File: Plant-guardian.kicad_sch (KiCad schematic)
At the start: 6 parts

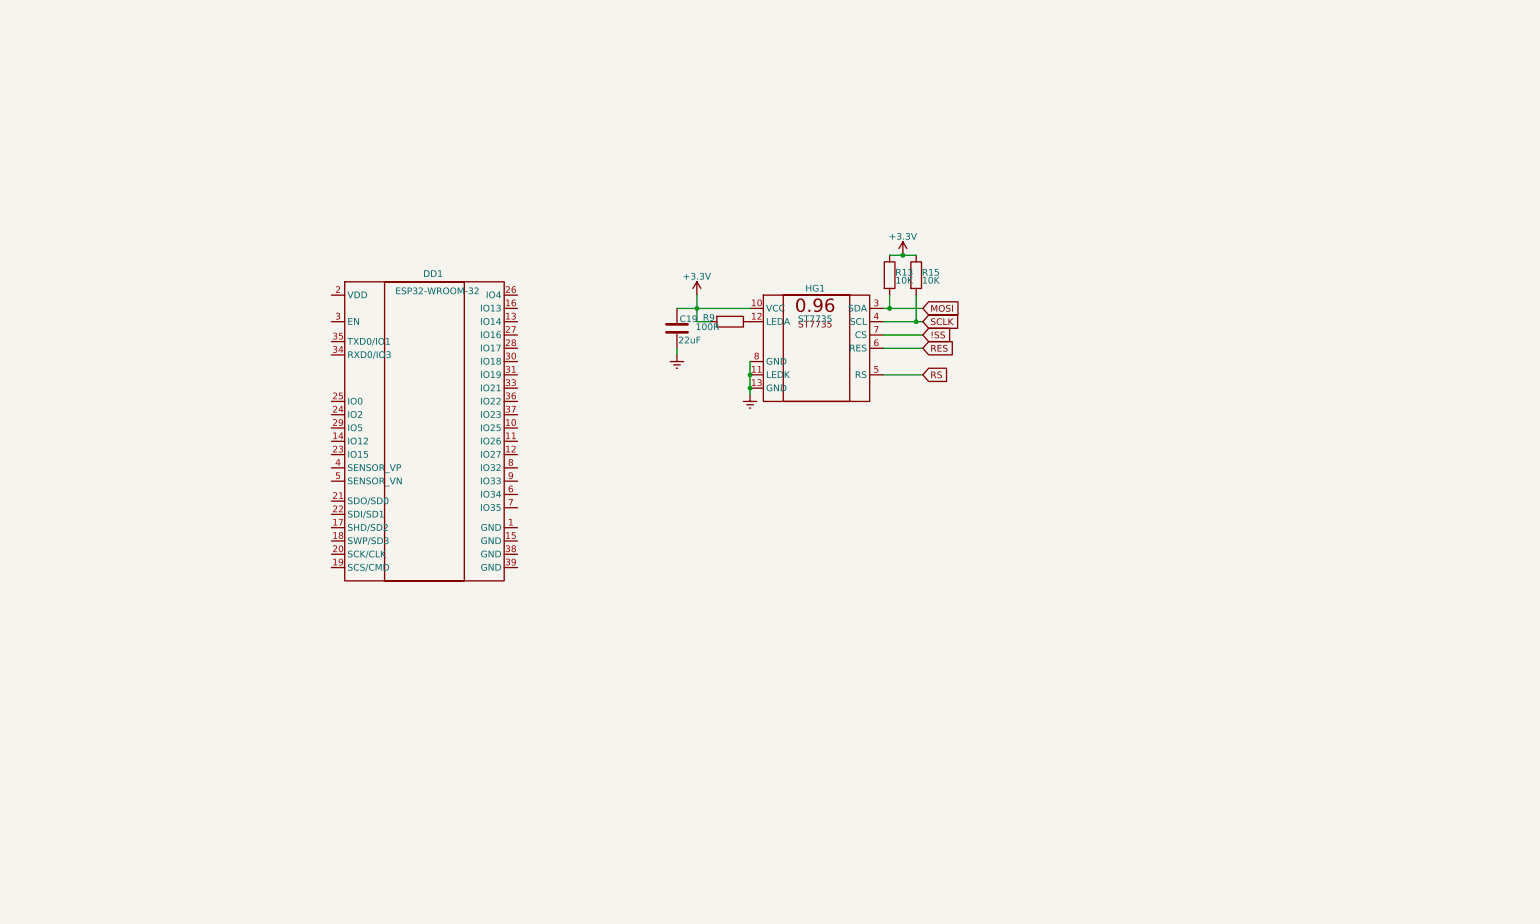
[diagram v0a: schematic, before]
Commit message: upd sch
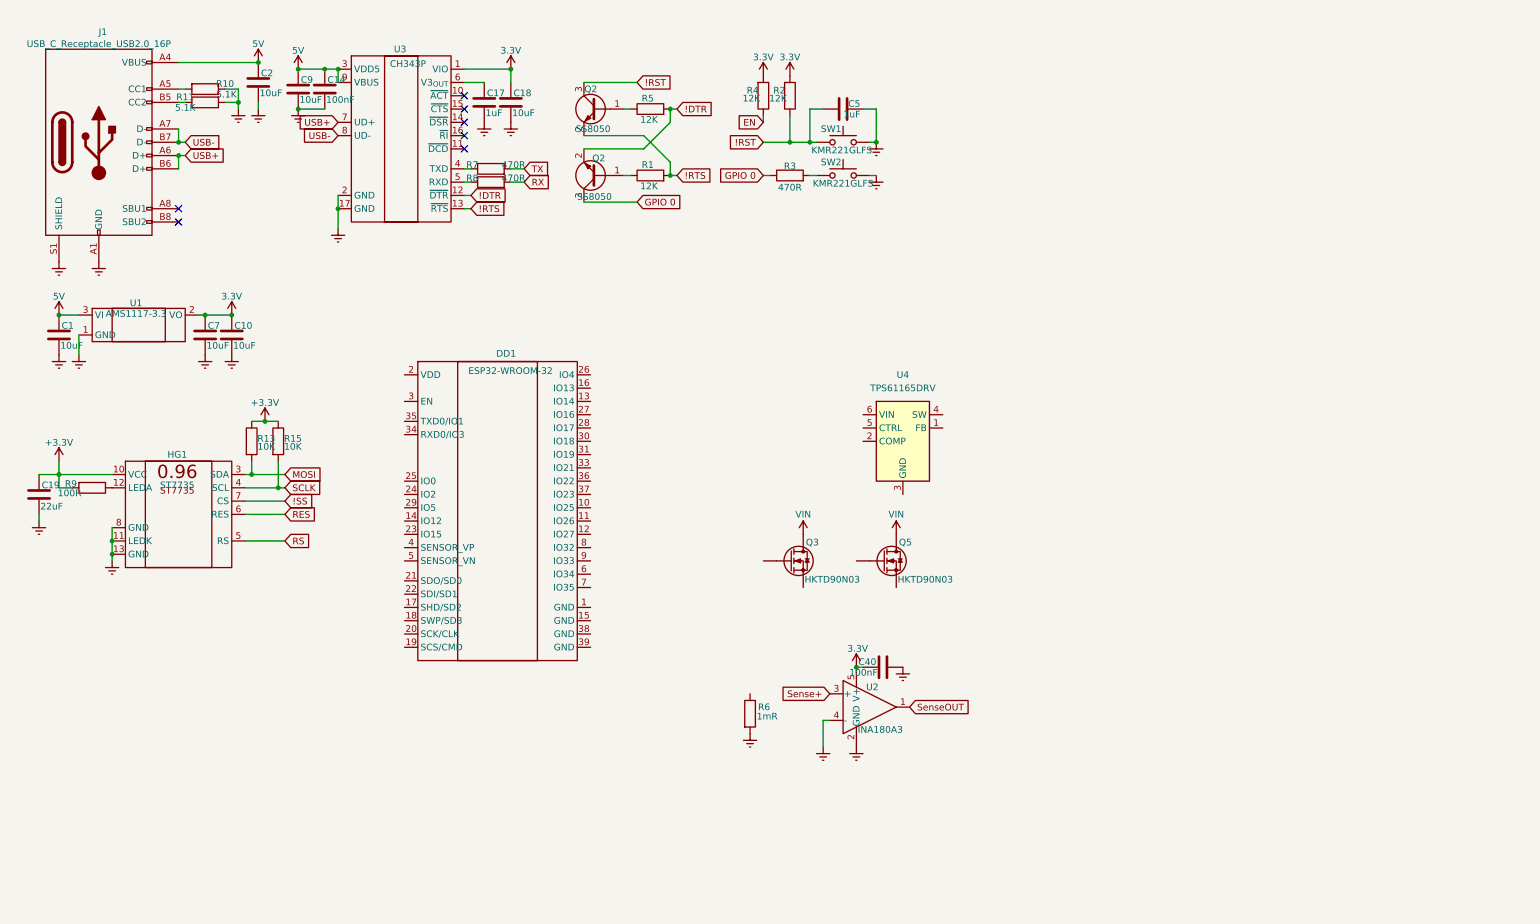
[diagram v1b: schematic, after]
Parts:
- added C1, C10, C18, C2, C7, C9: 10uF, Capacitor_SMD:C_0402_1005Metric, symbol Device:C
- added C14, C40: 100nF, Capacitor_SMD:C_0402_1005Metric, symbol Device:C
- added C17, C5: 1uF, Capacitor_SMD:C_0402_1005Metric, symbol Device:C
- added J1: USB_C_Receptacle_USB2.0_16P, Connector_USB:USB_C_Receptacle_GCT_USB4105-xx-A_16P_TopMnt_Horizontal, symbol Connector:USB_C_Receptacle_USB2.0_16P
- added Q2 (x2): SS8050, Package_TO_SOT_SMD:SOT-23, symbol Transistor_BJT:SS8050
- added Q3, Q5: HKTD90N03, Package_TO_SOT_SMD:TO-252-2, symbol Device:Q_NMOS
- added R1, R2, R4, R5: 12K, PCM_Resistor_SMD_AKL:R_0402_1005Metric, symbol Device:R
- added R10, R11: 5.1K, PCM_Resistor_SMD_AKL:R_0402_1005Metric, symbol Device:R
- added R3, R7, R8: 470R, PCM_Resistor_SMD_AKL:R_0402_1005Metric, symbol Device:R
- added R6: 1mR, PCM_Resistor_SMD_AKL:R_2512_6332Metric_Pad1.52x3.35mm, symbol Device:R
- added SW1, SW2: KMR221GLFS, Button_Switch_SMD:SW_SPST_PTS810, symbol Switch:SW_Push
- added U1: AMS1117-3.3, Package_TO_SOT_SMD:SOT-89-3, symbol Regulator_Linear:AMS1117-3.3
- added U2: INA180A3, Package_TO_SOT_SMD:SOT-23-5, symbol Amplifier_Current:INA180A1
- added U3: CH343P, Package_DFN_QFN:WCH_QFN-16-1EP_3x3mm_P0.5mm_EP1.8x1.8mm, symbol Interface_USB:CH343P
- added U4: TPS61165DRV, Package_SON:WSON-6-1EP_2x2mm_P0.65mm_EP1x1.6mm, symbol Driver_LED:TPS61165DRV
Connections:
- net Earth: now also C1.2, C10.2, C14.2, C17.2, C18.2, C2.2, C40.2, C5.2, C7.2, C9.2, J1.A1 (GND), J1.A12 (GND), J1.B1 (GND), J1.B12 (GND), J1.S1 (SHIELD), R10.1, R11.2, R6.2, SW1.1, SW2.1, U1.1 (GND), U2.2 (GND), U2.4 (-), U3.17 (GND), U3.2 (GND)
- new net: R7.1, U3.4 (TXD)
- new net: Q2.1 (B), R5.1
- new net: R3.2, SW2.2
- new net: J1.B5 (CC2), R11.1
- new net: C17.1, U3.6 (V3_{OUT})
- new net: R8.1, U3.5 (RXD)
- new net: J1.A5 (CC1), R10.2
- new net: U4.3 (GND), U4.7 (GND)
- new net: Q2.1 (B), R1.1
- new net !DTR: Q2.2 (E), R5.2, U3.12 (~{DTR})
- new net !RST: C5.1, Q2.3 (C), R2.1, SW1.2
- new net !RTS: Q2.2 (E), R1.2, U3.13 (~{RTS})
- new net 3.3V: C10.1, C18.1, C40.1, C7.1, R2.2, R4.2, U1.2 (VO), U2.5 (V+), U3.1 (VIO)
- new net 5V: C1.1, C14.1, C2.1, C9.1, J1.A4 (VBUS), J1.A9 (VBUS), J1.B4 (VBUS), J1.B9 (VBUS), U1.3 (VI), U3.3 (VDD5), U3.9 (VBUS)
- new net EN: R4.1
- new net GPIO 0: Q2.3 (C), R3.1
- new net RX: R8.2
- new net Sense+: U2.3 (+)
- new net SenseOUT: U2.1
- new net TX: R7.2
- new net USB+: J1.A6 (D+), J1.B6 (D+), U3.7 (UD+)
- new net USB-: J1.A7 (D-), J1.B7 (D-), U3.8 (UD-)
- new net VIN: Q3.2 (D), Q5.2 (D)
- no-connect marks 0 -> 7
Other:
- moved on the sheet: C19, DD1, HG1, R13, R15, R9

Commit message: schematics done, placement on PCB done
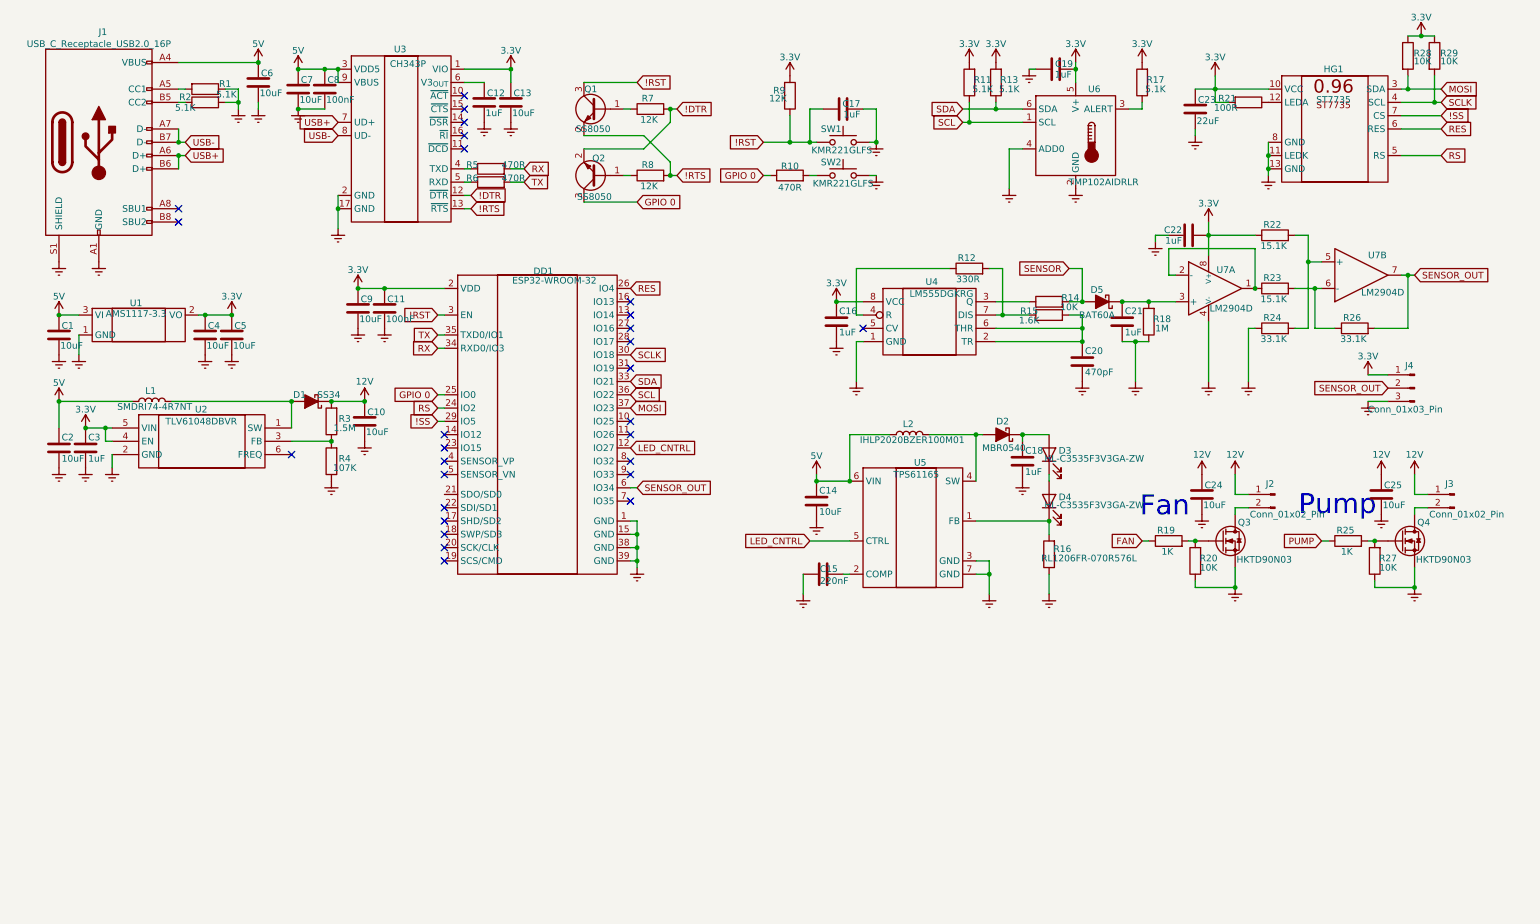
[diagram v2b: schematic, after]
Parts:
- removed C40: 100nF, Capacitor_SMD:C_0402_1005Metric, symbol Device:C
- removed Q5: HKTD90N03, Package_TO_SOT_SMD:TO-252-2, symbol Device:Q_NMOS
- removed R6: 1mR, PCM_Resistor_SMD_AKL:R_2512_6332Metric_Pad1.52x3.35mm, symbol Device:R
- removed U2: INA180A3, Package_TO_SOT_SMD:SOT-23-5, symbol Amplifier_Current:INA180A1
- added C10, C14, C2, C24, C25, C9: 10uF, Capacitor_SMD:C_0402_1005Metric, symbol Device:C
- added C11: 100nF, Capacitor_SMD:C_0402_1005Metric, symbol Device:C
- added C15: 220nF, Capacitor_SMD:C_0402_1005Metric, symbol Device:C
- added C16, C18, C19, C21, C22, C3: 1uF, Capacitor_SMD:C_0402_1005Metric, symbol Device:C
- added C20: 470pF, Capacitor_SMD:C_0402_1005Metric, symbol Device:C
- added D1: SS34, PCM_Diode_SMD_AKL:D_SMC, symbol PCM_Diode_Schottky_AKL:SS34
- added D2: MBR0540, PCM_Diode_SMD_AKL:D_SOD-123, symbol PCM_Diode_Schottky_AKL:MBR0540
- added D3, D4: HL-C3535F3V3GA-ZW, SMD3535-3P:SMD3535-3P, symbol Device:LED
- added D5: BAT60A, PCM_Diode_SMD_AKL:D_SOD-323, symbol PCM_Diode_Schottky_AKL:BAT60A
- added J2, J3: Conn_01x02_Pin, Connector_PinHeader_2.54mm:PinHeader_1x02_P2.54mm_Vertical, symbol Connector:Conn_01x02_Pin
- added J4: Conn_01x03_Pin, Connector_PinHeader_2.54mm:PinHeader_1x03_P2.54mm_Vertical, symbol Connector:Conn_01x03_Pin
- added L1: SMDRI74-4R7NT, Inductor_SMD:L_SXN_SMDRI73, symbol Device:L
- added L2: IHLP2020BZER100M01, Inductor_SMD:L_APV_APH0518, symbol Device:L
- added Q4: HKTD90N03, Package_TO_SOT_SMD:TO-252-2, symbol Device:Q_NMOS
- added R11, R13, R17: 5.1K, PCM_Resistor_SMD_AKL:R_0402_1005Metric, symbol Device:R
- added R12: 330R, PCM_Resistor_SMD_AKL:R_0402_1005Metric, symbol Device:R
- added R14, R20, R27: 10K, PCM_Resistor_SMD_AKL:R_0402_1005Metric, symbol Device:R
- added R15: 1.6K, PCM_Resistor_SMD_AKL:R_0402_1005Metric, symbol Device:R
- added R16: RL1206FR-070R576L, Resistor_SMD:R_1206_3216Metric, symbol Device:R
- added R18: 1M, PCM_Resistor_SMD_AKL:R_0402_1005Metric, symbol Device:R
- added R19, R25: 1K, PCM_Resistor_SMD_AKL:R_0402_1005Metric, symbol Device:R
- added R22, R23: 15.1K, PCM_Resistor_SMD_AKL:R_0402_1005Metric, symbol Device:R
- added R24, R26: 33.1K, PCM_Resistor_SMD_AKL:R_0402_1005Metric, symbol Device:R
- added R3: 1.5M, PCM_Resistor_SMD_AKL:R_0402_1005Metric, symbol Device:R
- added U2: TLV61048DBVR, PCM_Package_TO_SOT_SMD_AKL:SOT-23-6, symbol TLV61048DBVR:TLV61048DBVR
- added U4: LM555DGKRG, Package_SO:VSSOP-8_3x3mm_P0.65mm, symbol Timer:LMC555xMM
- added U6: TMP102AIDRLR, Package_TO_SOT_SMD:SOT-563, symbol Sensor_Temperature:TMP102xxDRL
- added U7: LM2904D, Package_SO:SOIC-8_5.3x6.2mm_P1.27mm, symbol PCM_Amplifier_Operational_AKL:LM2904D
- R4: value 12K -> 107K
- U5: renamed from U4; value TPS61165DRV -> TPS61165
- renumbered C17 to C12, C18 to C13, C5 to C17, C19 to C23, C7 to C4, C10 to C5, C2 to C6, C9 to C7, C14 to C8, Q2 to Q1, R10 to R1, R3 to R10, R11 to R2, R9 to R21, R13 to R28, R15 to R29, R7 to R5, R8 to R6, R5 to R7, R1 to R8, R2 to R9
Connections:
- net +3.3V is gone; now on net 3.3V: C23.1, HG1.10 (VCC), R21.2, R28.1, R29.1
- net EN is gone; now on net Earth: R4.1
- net !RST: now also DD1.3 (EN)
- net !SS: now also DD1.29 (IO5)
- net 3.3V: now also DD1.2 (VDD), C11.1, C16.2, C19.2, C22.2, C3.2, C9.1, J4.1 (Pin_1), R11.2, R13.2, R17.2, R22.1, U2.4 (EN), U2.5 (VIN), U4.8 (VCC), U6.5 (V+), U7.8 (V+); no longer R4.2
- net 5V: now also U5.6 (VIN), C14.2, C2.2, L1.1, L2.1
- net Earth: now also DD1.1 (GND), DD1.15 (GND), DD1.38 (GND), DD1.39 (GND), Q3.3 (S), U5.3 (GND), U5.7 (GND), C10.2, C11.2, C14.1, C15.1, C16.1, C18.1, C19.1, C2.1, C20.1, C21.1, C22.1, C24.2, C25.2, C3.1, C9.2, J4.3 (Pin_3), Q4.3 (S), R16.1, R18.1, R20.1, R24.1, R27.1, U2.2 (GND), U4.1 (GND), U6.2 (GND), U6.4 (ADD0), U7.4 (V-)
- net GPIO 0: now also DD1.25 (IO0)
- net MOSI: now also DD1.37 (IO23)
- net RES: now also DD1.26 (IO4)
- net RS: now also DD1.24 (IO2)
- net RX: now also DD1.34 (RXD0/IO3), R5.2; no longer R6.2
- net SCLK: now also DD1.30 (IO18)
- net TX: now also DD1.35 (TXD0/IO1), R6.2; no longer R5.2
- net at U5.1 (FB): now also D4.1 (K), R16.2
- net at U5.2 (COMP): now also C15.2
- net at U5.4 (SW): now also D2.2 (A), L2.2
- net LED_CNTRL: now reaches U5.5 (CTRL)
- net LED_CNTRL: now also DD1.12 (IO27)
- net at Q3.1 (G): now also R19.2, R20.2
- net SDA: now reaches DD1.33 (IO21)
- net SDA: now also R13.1, U6.6 (SDA)
- net SCL: now reaches DD1.36 (IO22)
- net SCL: now also R11.1, U6.1 (SCL)
- net SENSOR_OUT: now reaches DD1.6 (IO34)
- net SENSOR_OUT: now also J4.2 (Pin_2), R26.2, U7.7
- net VIN: no longer names the net of Q3.2 (D)
- net VIN: now also J2.2 (Pin_2)
- new net: R3.1, R4.2, U2.3 (FB)
- new net: R17.1, U6.3 (ALERT)
- new net: D3.1 (K), D4.2 (A)
- new net: C18.2, D2.1 (K), D3.2 (A)
- new net: C21.2, D5.1 (K), R18.2, U7.3 (+)
- new net: C20.2, R15.2, U4.2 (TR), U4.6 (THR)
- new net: D1.2 (A), L1.2, U2.1 (SW)
- new net: R23.1, U7.1, U7.2 (-)
- new net: R23.2, R26.1, U7.6 (-)
- new net: Q4.1 (G), R25.2, R27.2
- new net: J3.2 (Pin_2), Q4.2 (D)
- new net: R22.2, R24.2, U7.5 (+)
- new net: R14.1, U4.3 (Q)
- new net: R12.1, U4.4 (R)
- new net: R12.2, R15.1, U4.7 (DIS)
- new net 12V: C10.1, C24.1, C25.1, D1.1 (K), J2.1 (Pin_1), J3.1 (Pin_1), R3.2
- new net FAN: R19.1
- new net PUMP: R25.1
- new net SENSOR: D5.2 (A), R14.2
- no-connect marks 7 -> 28
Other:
- note added: "Fan"
- note added: "Pump"
- moved on the sheet: C23, DD1, HG1, Q3, R21, R28, R29

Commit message: rev0 ready
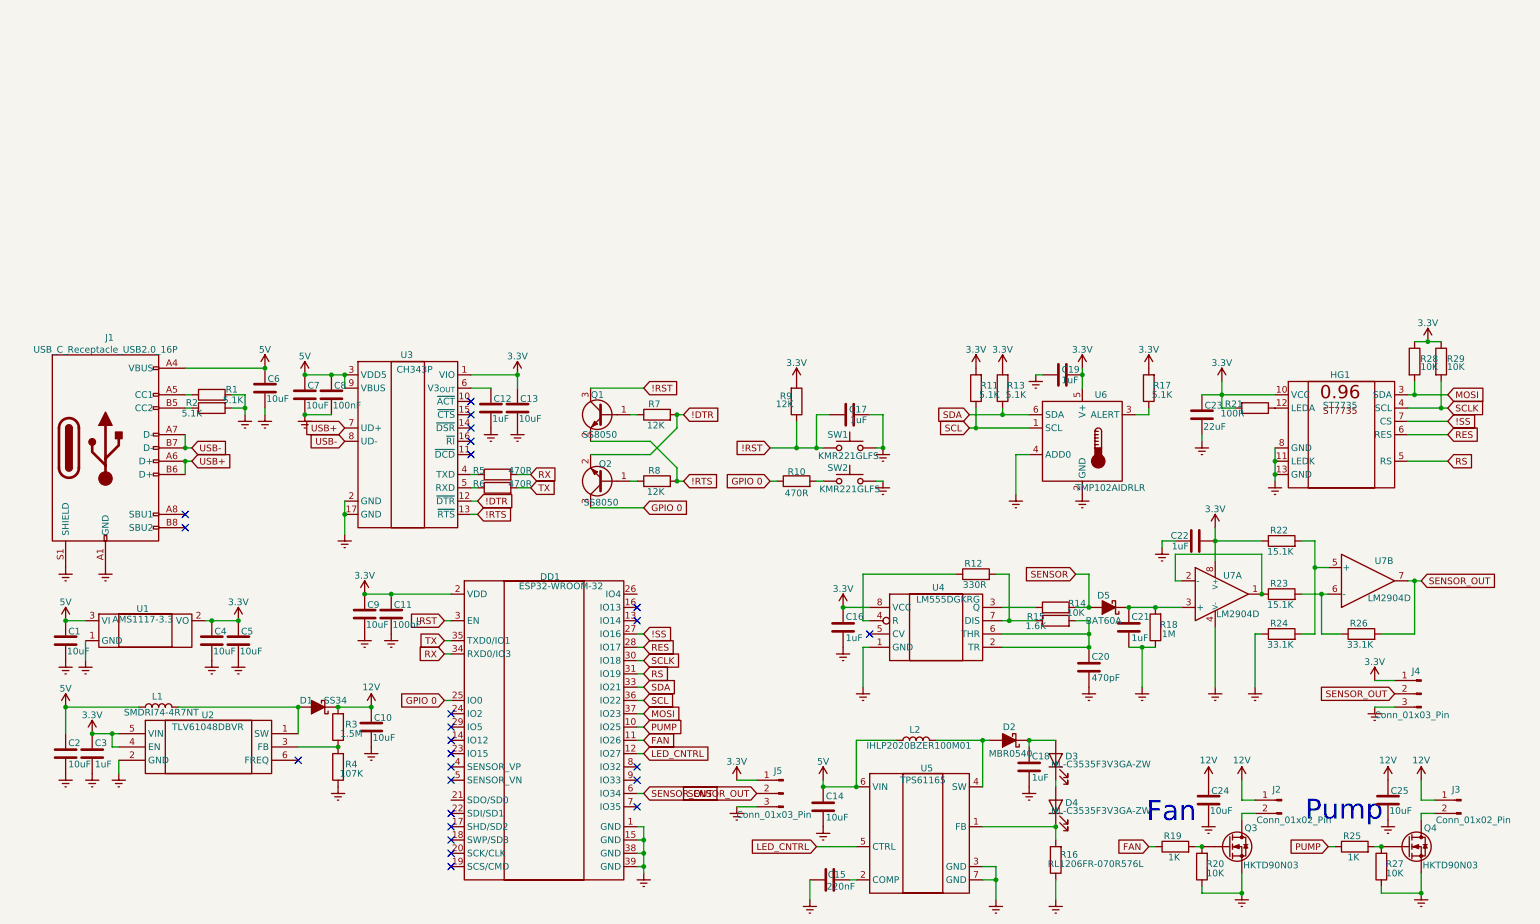
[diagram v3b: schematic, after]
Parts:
- added J5: Conn_01x03_Pin, Connector_PinHeader_2.54mm:PinHeader_1x03_P2.54mm_Vertical, symbol Connector:Conn_01x03_Pin
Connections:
- net !SS: now also DD1.27 (IO16); no longer DD1.29 (IO5)
- net 3.3V: now also J5.1 (Pin_1)
- net Earth: now also J5.3 (Pin_3)
- net FAN: now also DD1.11 (IO26)
- net PUMP: now also DD1.10 (IO25)
- net RES: now also DD1.28 (IO17); no longer DD1.26 (IO4)
- net RS: now also DD1.31 (IO19); no longer DD1.24 (IO2)
- net SENSOR_OUT: now also J5.2 (Pin_2)
- no-connect marks 28 -> 25
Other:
- moved on the sheet: C1, C10, C11, C12, C13, C14, C15, C16, C17, C18, C19, C2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
